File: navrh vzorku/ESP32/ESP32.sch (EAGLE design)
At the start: 20 parts, among them U1 ESP-WROOM-32

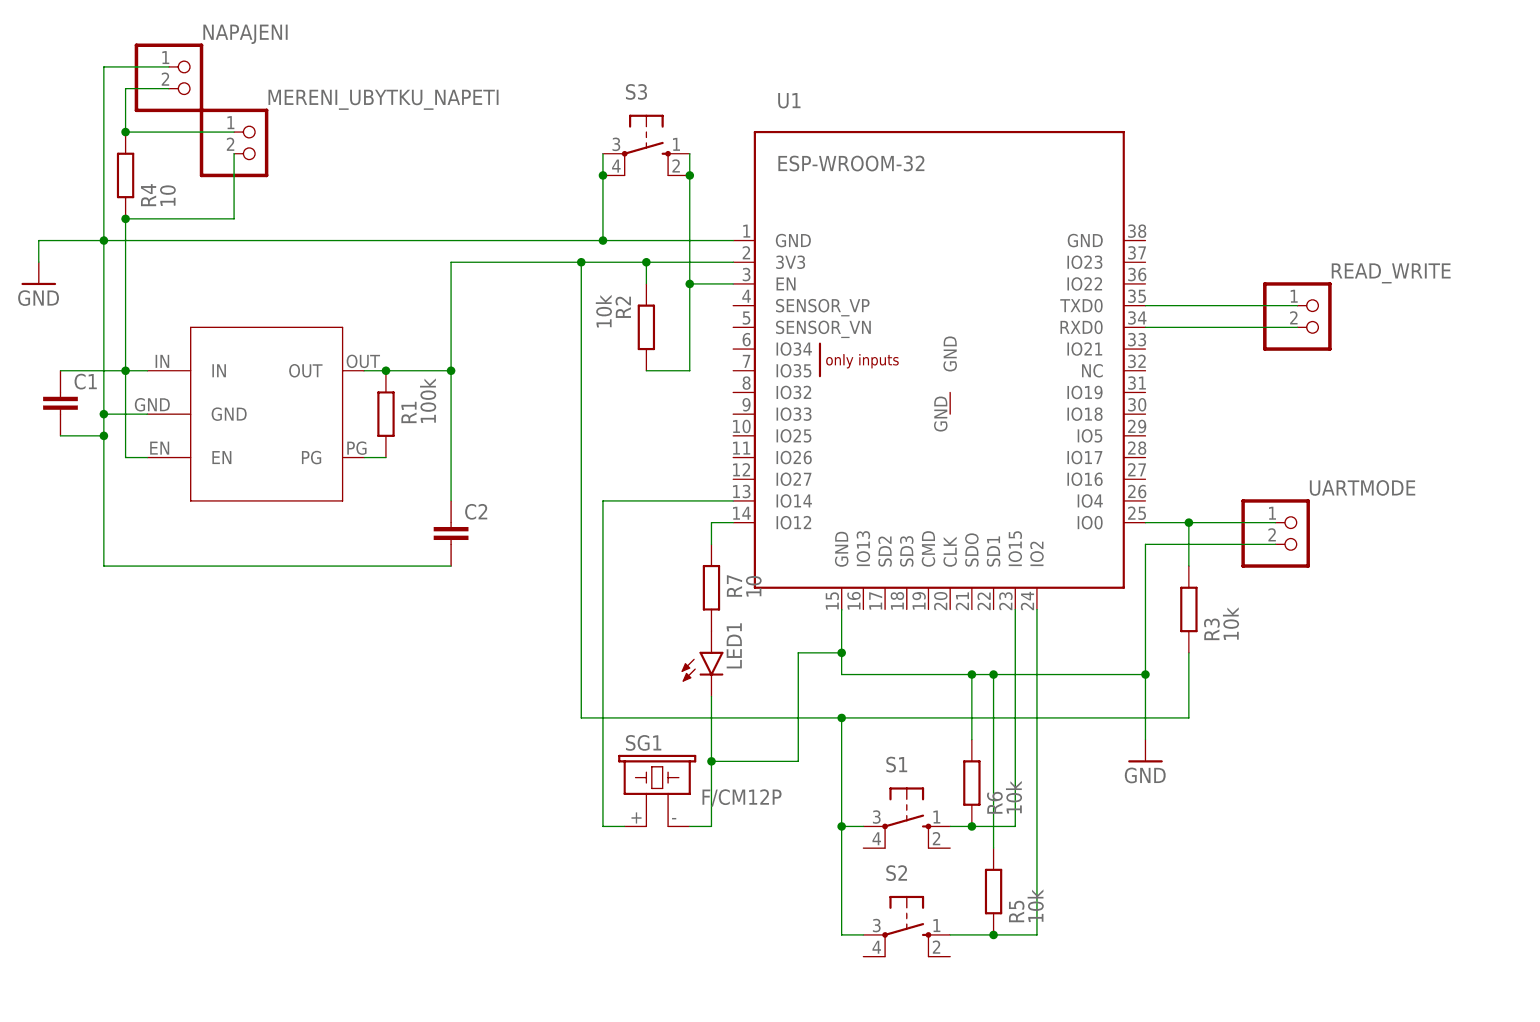
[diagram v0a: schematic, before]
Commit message: Finalni verze
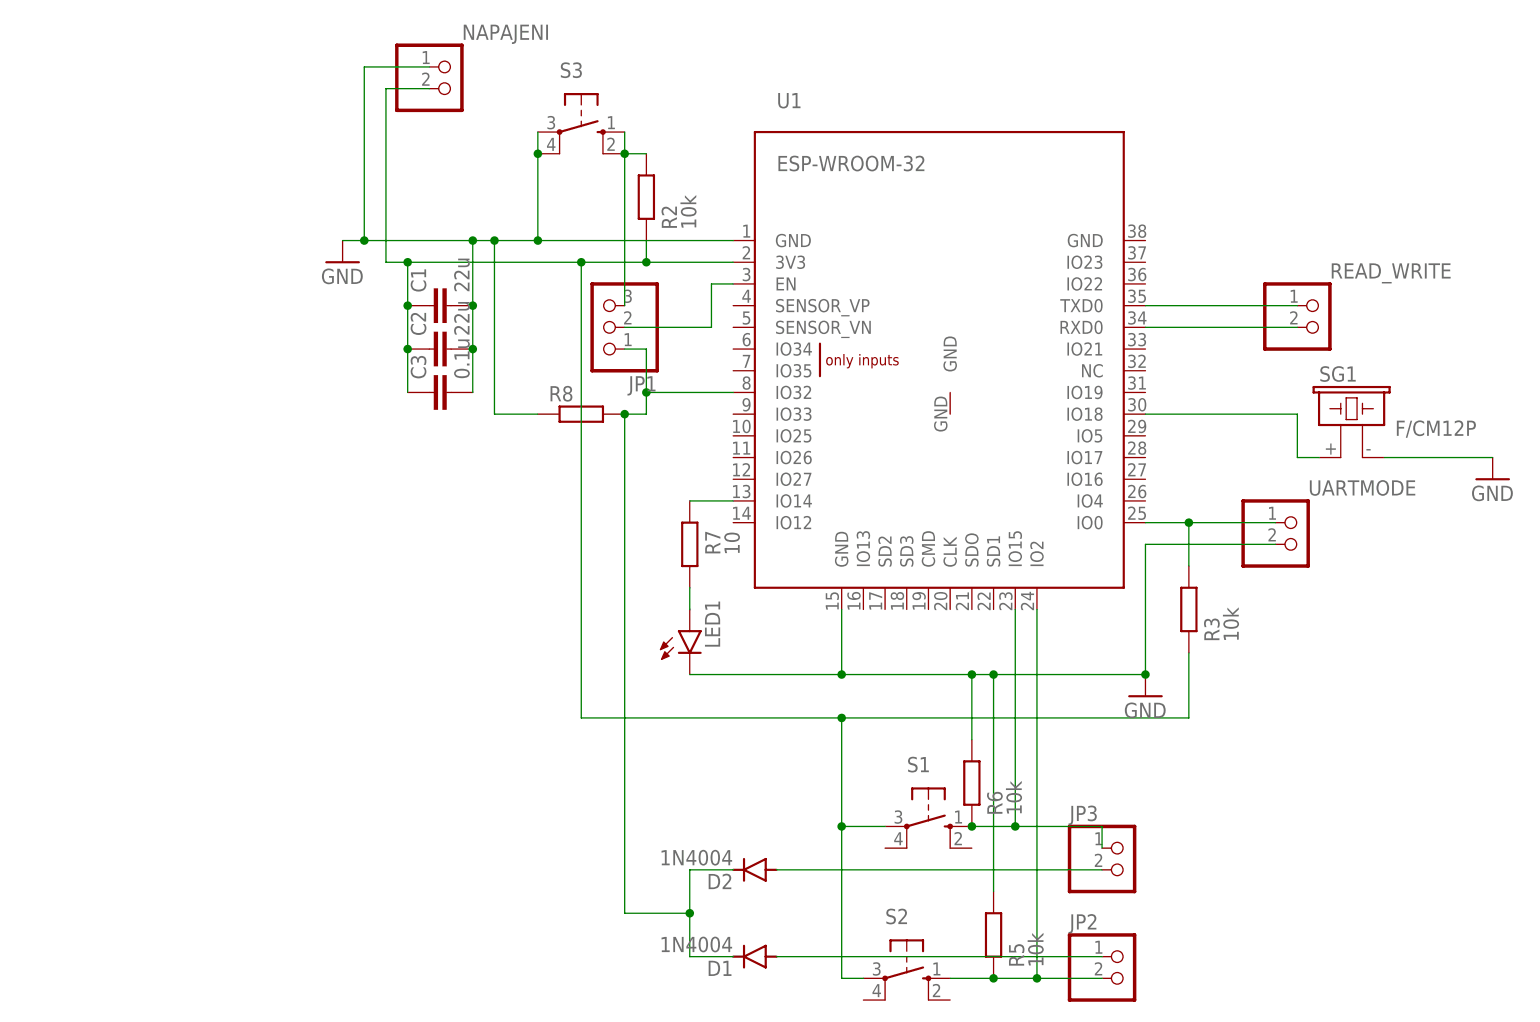
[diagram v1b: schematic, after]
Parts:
- removed MERENI_UBYTKU_NAPETI: (no value), pinhead:PINHD-1X2
- removed R1: 100k, rcl:R-EU_0207/10
- removed R4: 10, rcl:R-EU_0207/10
- removed U$1: LDLN030, WT8266:LDLN030
- added C3: 0.1u, capacitor-wima:C2.5/2
- added D1, D2: 1N4004, diode:1N4004
- added JP1: (no value), pinhead:PINHD-1X3
- added JP2, JP3: (no value), pinhead:PINHD-1X2
- added R8: (no value), rcl:R-EU_0207/10
- C1, C2: value (none) -> 22u
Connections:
- removed net N$10: MERENI_UBYTKU_NAPETI.1, NAPAJENI.2, R4.2
- removed net N$4: R1.1, U$1.PG
- removed net N$9: R7.2, U1.IO12
- new net N$15: D1.C, D2.C, JP1.1, R8.2, U1.IO32
- new net N$17: D1.A, JP2.1
- new net N$18: D2.A, JP3.2
- new net N$3: JP1.3, R2.2, S3.S, S3.S1
- net GND: now also C3.2, R8.1; no longer U$1.GND
- net N$1: now also SG1.1, U1.IO18; no longer C1.1, MERENI_UBYTKU_NAPETI.2, R4.1, U$1.EN, U$1.IN
- net N$11: now also JP2.2
- net N$12: now also JP3.1
- net N$13: now also R7.2; no longer SG1.1
- net N$2: now also C1.1, C3.1, NAPAJENI.2; no longer R1.2, U$1.OUT
- net N$5: now also JP1.2; no longer R2.2, S3.S, S3.S1
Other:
- moved on the sheet: C1, C2, LED1, NAPAJENI, R2, R5, R7, S1, S2, S3, SG1
